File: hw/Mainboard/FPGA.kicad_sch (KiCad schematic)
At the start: 57 parts, among them J5 PMOD1, J6 PMOD2, J7 PROG, J8 FPGA_MCU, J9 BUS_EXPANSION, Q1 MMBT3904, SW3 CONFIG, U10 T8Q144C3

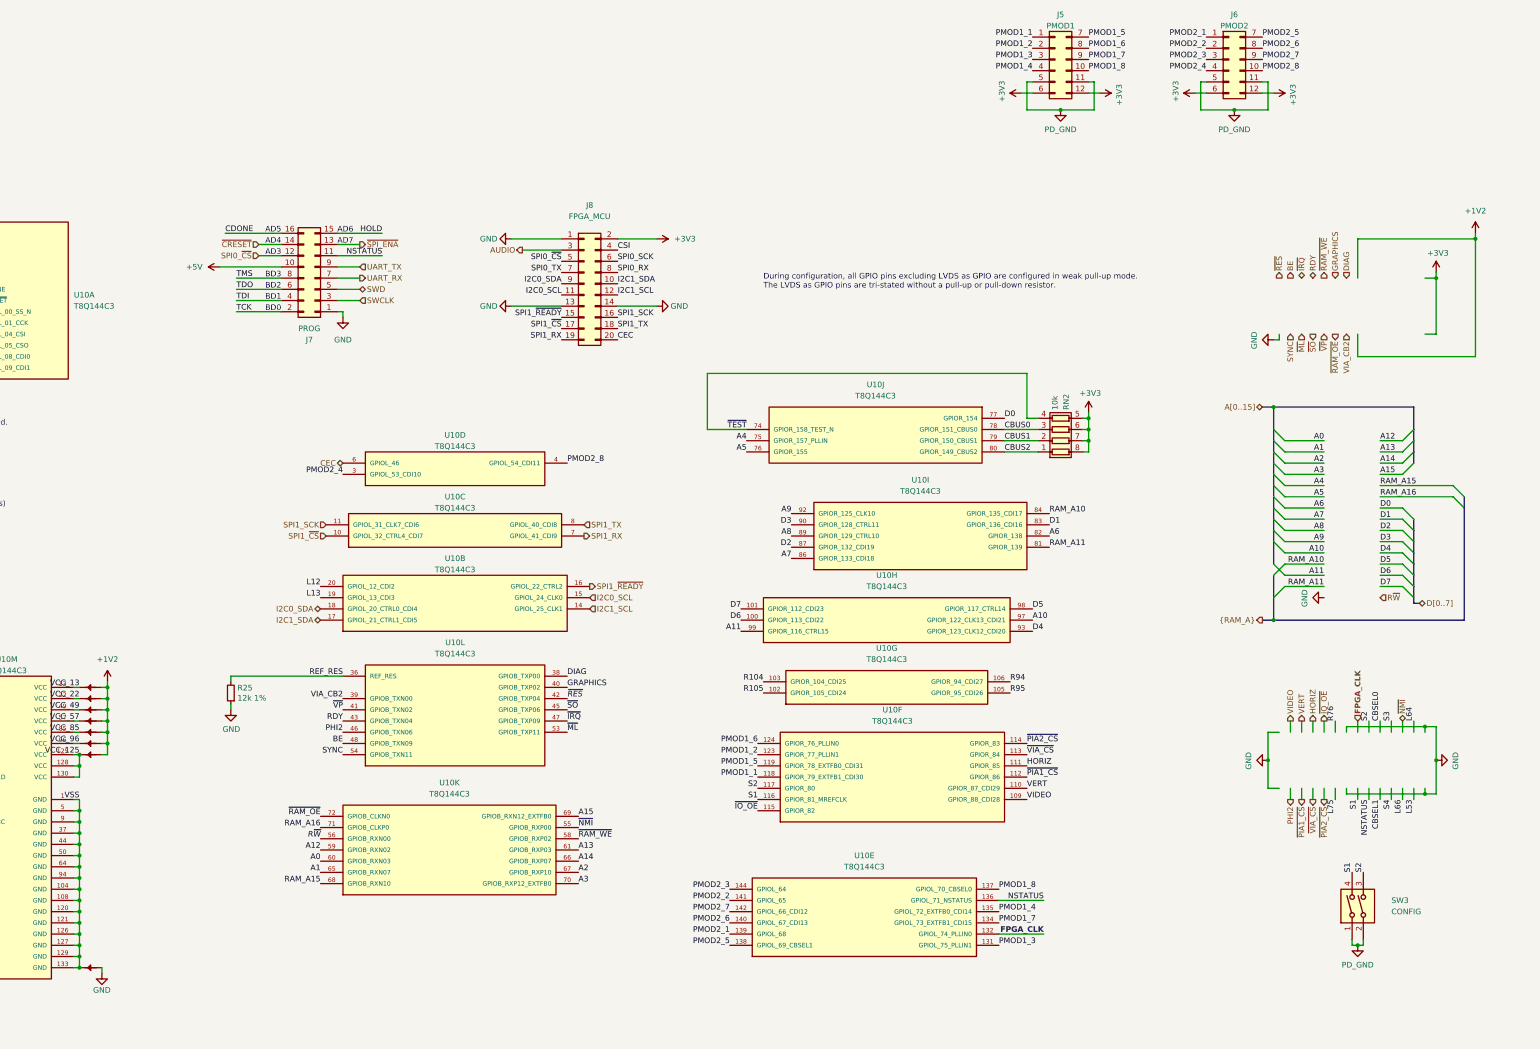
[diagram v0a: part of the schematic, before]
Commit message: hw: fill, routing, and silk touchups (wip)
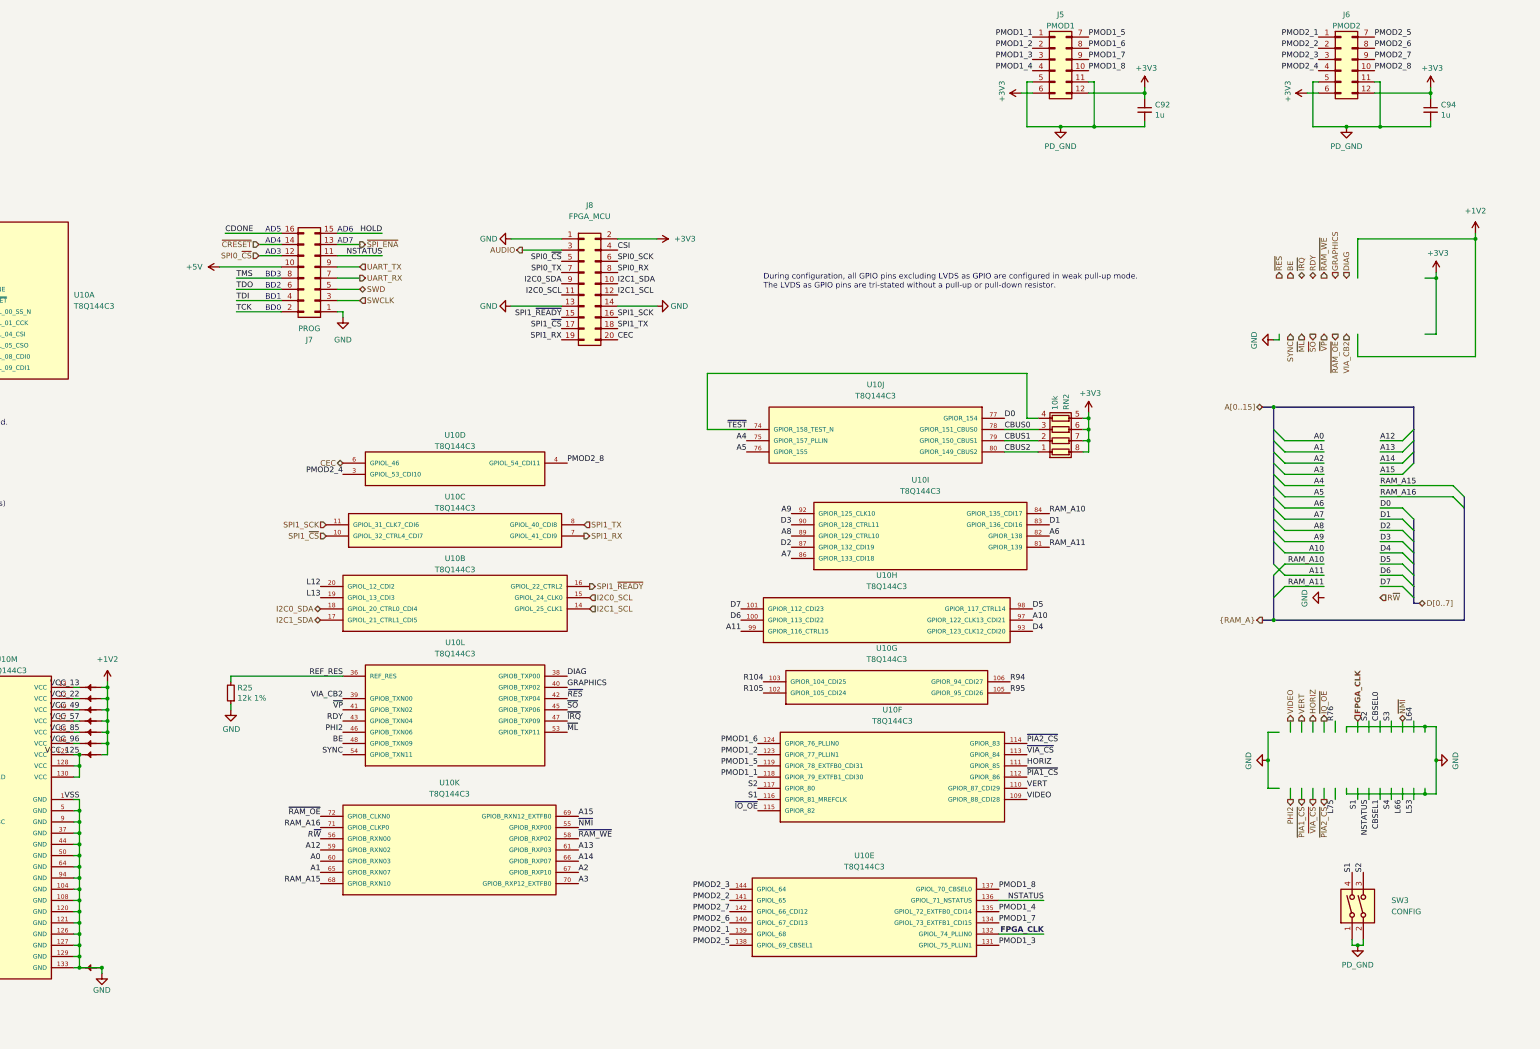
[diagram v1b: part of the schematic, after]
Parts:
- added C92, C94: 1u, Capacitor_SMD:C_0402_1005Metric, symbol Device:C_Small
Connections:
- net VSS is gone; now on net GND: PT30.2, U10.1 (GND), U10.104 (GND), U10.108 (GND), U10.120 (GND), U10.121 (GND), U10.126 (GND), U10.127 (GND), U10.129 (GND), U10.133 (GND), U10.37 (GND), U10.44 (GND), U10.5 (GND), U10.50 (GND), U10.64 (GND), U10.9 (GND), U10.94 (GND)
- net +3V3: now also C92.1, C94.1
- net PD_GND: now also C92.2, C94.2
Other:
- moved on the sheet: J6
